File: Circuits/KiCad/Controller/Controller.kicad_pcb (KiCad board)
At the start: 2 copper layers, 177.2 x 109.2 mm, 60 parts, among them J1 Conn_01x15_Male, J2 Conn_01x24_Male, J3 Conn_01x24_Male, U1 74x08, U10 W29C040, U11 74x138, U12 74x273, U13 74x273, U14 74x273, U15 74x273, U16 74x273, U17 74x273, U18 74x04, U19 74x04, U2 74x08, U20 74x32, U21 74x04, U22 74x04, U23 74x02, U24 74x02, U25 74x04, U27 74x161, U3 74x04, U4 74x27, U5 74x02, U6 74x161, U7 74x161, U8 74x161, U9 74x74, Y1 8 MHz (max. 10 MHz)

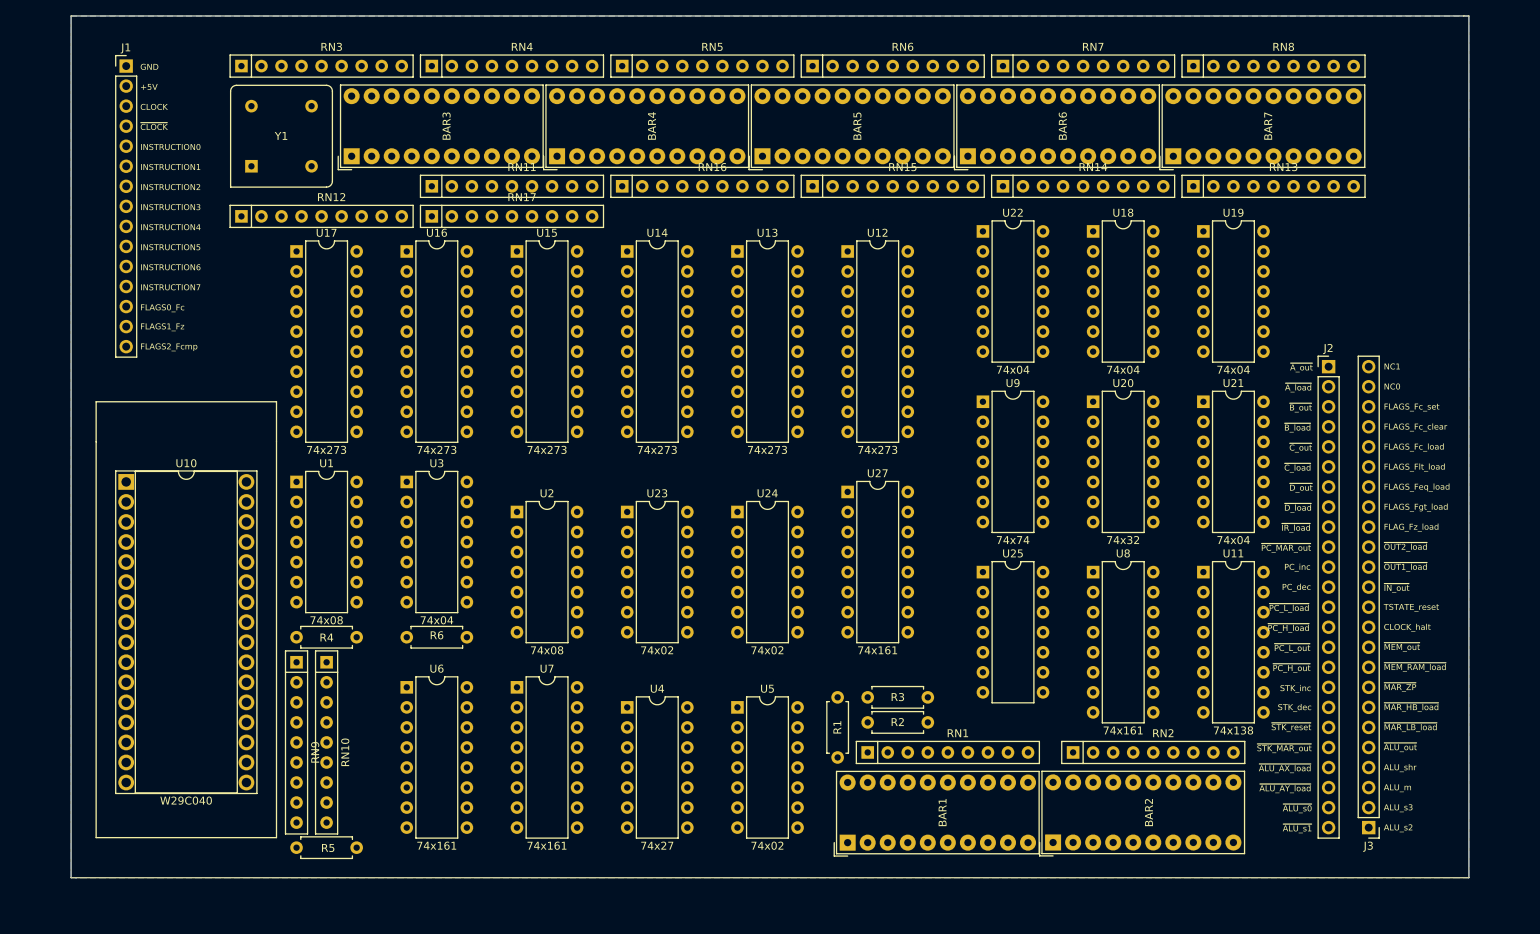
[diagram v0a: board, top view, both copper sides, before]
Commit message: Controller PCB rev2
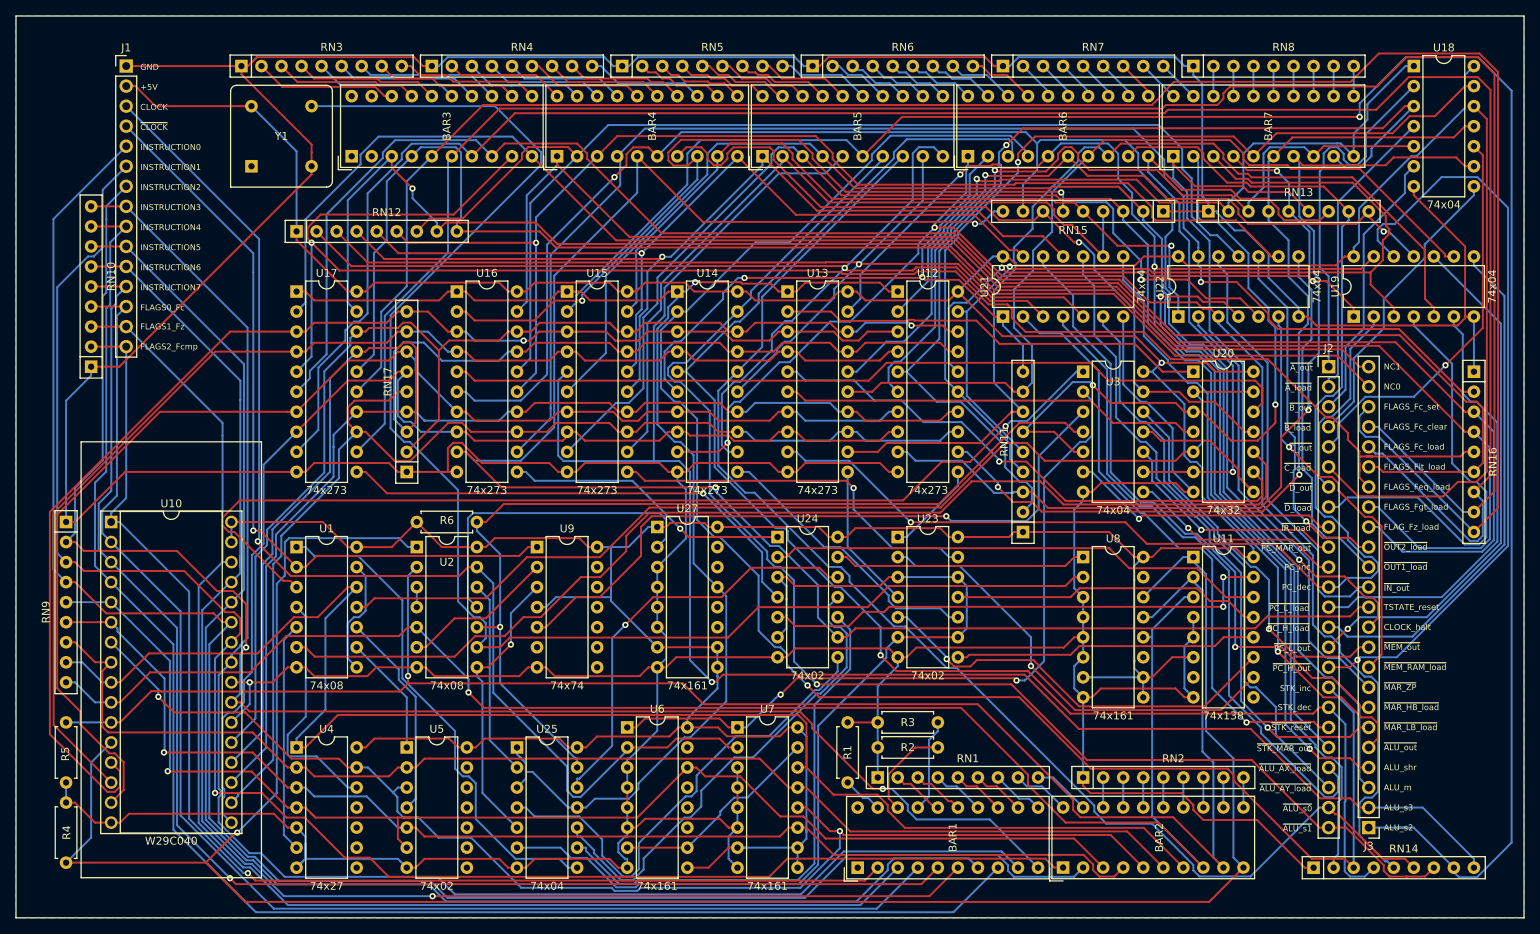
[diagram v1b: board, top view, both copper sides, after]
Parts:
- BAR1, BAR2, BAR3, BAR4, BAR5, BAR6, BAR7: footprint Display:HDSP-4830 -> 74xx-Computer-Footprints:Bar-Graph-10
- moved RN16 110.5 mm to (198.1, 71.8), turned to 270 degrees
- moved RN14 94.9 mm to (177.8, 134.6)
- moved U3 86.9 mm to (148.6, 71.8)
- moved RN11 86.8 mm to (141.0, 92.1), turned to 90 degrees
- moved U25 63.1 mm to (76.8, 119.4)
- moved U9 59.4 mm to (79.4, 94.0)
- moved RN10 47.9 mm to (22.9, 71.1), turned to 90 degrees
- moved U18 45.7 mm to (190.5, 33.0)
- moved RN15 44.6 mm to (158.8, 51.4), turned to 180 degrees
- moved U4 42.2 mm to (48.9, 119.4)
- moved U5 42.2 mm to (62.9, 119.4)
- moved R4 40.9 mm to (19.7, 134.0), turned to 90 degrees
- moved U23 34.4 mm to (125.1, 92.7)
- moved RN9 34.2 mm to (19.7, 90.8)
- moved R5 33.2 mm to (19.7, 116.2), turned to 270 degrees
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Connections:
- U10 pad 31: (no net) -> +5V
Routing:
- net GND: track 0.00 -> 881.3 mm, vias 0 -> 1
- net +5V: track 0.00 -> 604.4 mm, vias 0 -> 1
- net BANK0: track 0.00 -> 284.2 mm, vias 0 -> 1
- net FLAGS_Fc_load: track 0.00 -> 265.2 mm
- net ALU_s2: track 0.00 -> 260.7 mm, vias 0 -> 1
- net FLAGS_Fc_set: track 0.00 -> 258.3 mm
- net FLAGS_Fc_clear: track 0.00 -> 255.5 mm
- net TSTATE_reset: track 0.00 -> 233.4 mm, vias 0 -> 2
- net INSTRUCTION0: track 0.00 -> 228.0 mm
- net BANK1: track 0.00 -> 221.2 mm, vias 0 -> 1
- net INSTRUCTION1: track 0.00 -> 216.5 mm, vias 0 -> 1
- net ALU_s3: track 0.00 -> 216.2 mm, vias 0 -> 1
- net STK_inc: track 0.00 -> 216.0 mm, vias 0 -> 1
- net FLAGS_Feq_load: track 0.00 -> 215.7 mm, vias 0 -> 1
- net FLAGS_Fgt_load: track 0.00 -> 213.2 mm
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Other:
- board size 177.2 x 109.2 mm -> 191.1 x 114.3 mm
- net class Power: trace_width 0.35 -> 0.25
